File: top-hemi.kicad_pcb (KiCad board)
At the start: 2 copper layers, 46 x 39 mm, 37 parts, among them J1 USB_B_Mini, J2 TC2030_NL, J3 FFC-0.5MM-6POS, J4 Port_1, J5 Port_2, J6 FFC-0.5MM-6POS, J7 Port_3, J8 Port_4, U1 PMIC-LDO-XC6204B332MR_SOT23-5_, U2 LP2985-5.0, U3 ATmega328P-MU, U4 ADXL335, Y1 16MHz

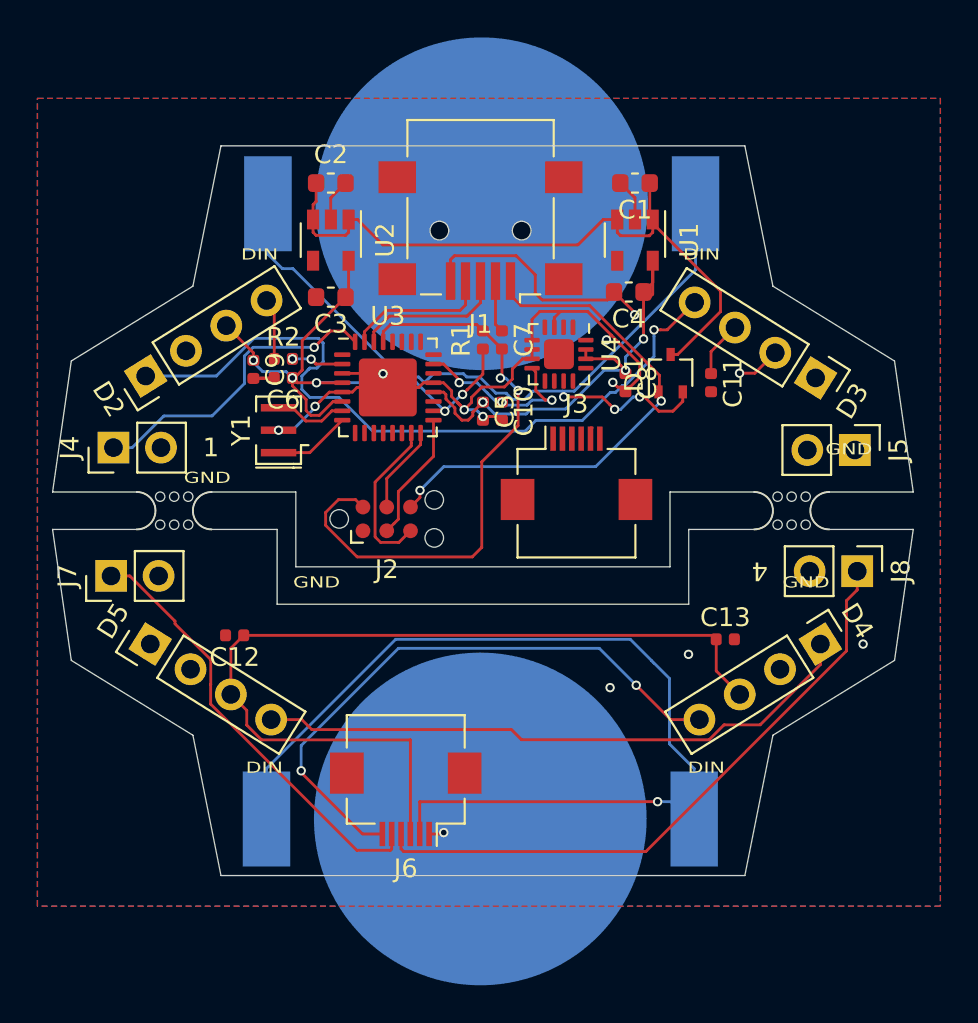
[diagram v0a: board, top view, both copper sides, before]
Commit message: Finish routing top board
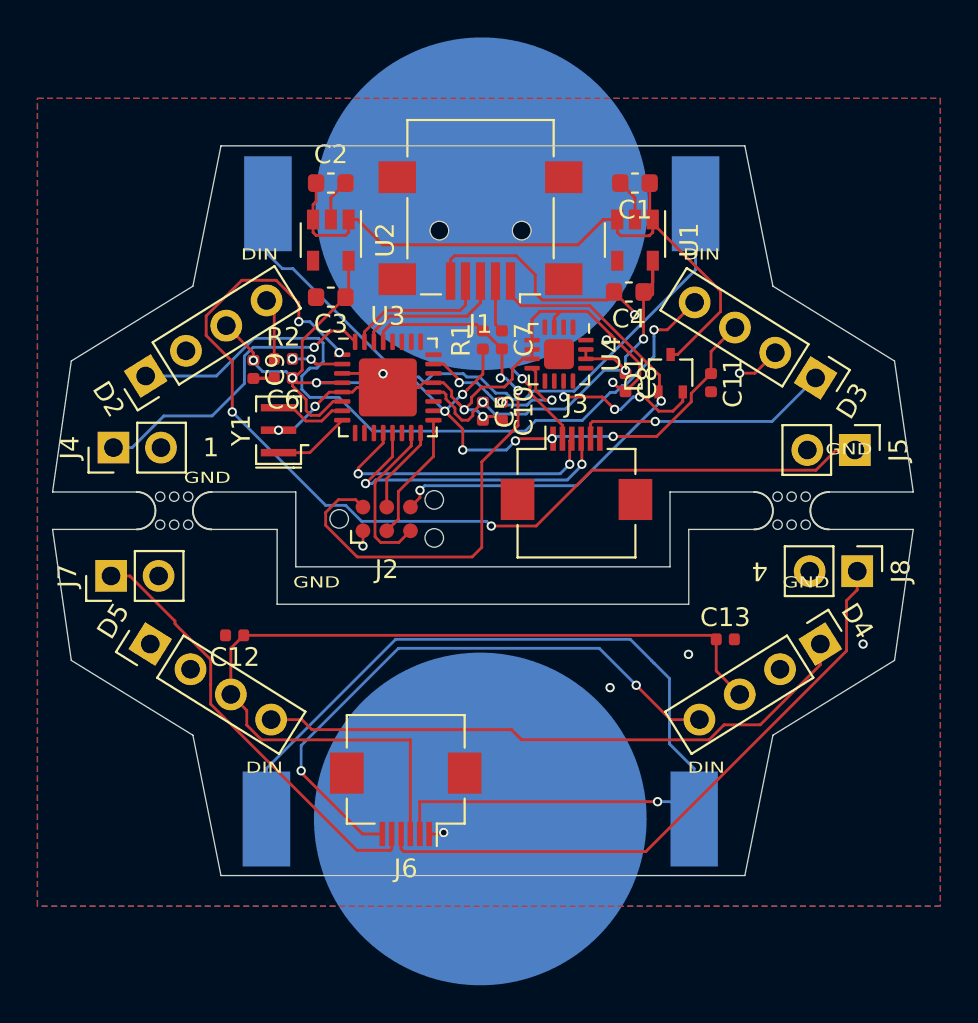
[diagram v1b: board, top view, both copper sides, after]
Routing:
- net /Top Hemisphere/BNC-2: track 0.00 -> 53.5 mm, vias 0 -> 4
- net +5V: track 84.0 -> 101.7 mm, vias 5 -> 9
- net /Top Hemisphere/BNC-4: track 0.00 -> 16.7 mm, vias 0 -> 2
- net /Top Hemisphere/BNC-3: track 0.00 -> 15.7 mm, vias 0 -> 2
- net /Top Hemisphere/BATT-BOT: track 6.12 -> 20.5 mm, vias 0 -> 1
- net /Top Hemisphere/DOUT-BOT: track 0.08 -> 13.9 mm, vias 0 -> 1
- net GND: track 57.7 -> 58.5 mm, vias 13 -> 14
